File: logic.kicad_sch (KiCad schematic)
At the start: 41 parts, among them J4 Conn_01x04, J5 Conn_01x04, J6 Conn_01x04_Pin, J7 TC2030, SW1 SW_Push, SW2 SW_Push, U6 SN65HVD230, U7 HT753-1, U8 STM32F103C8Tx, Y1 8M

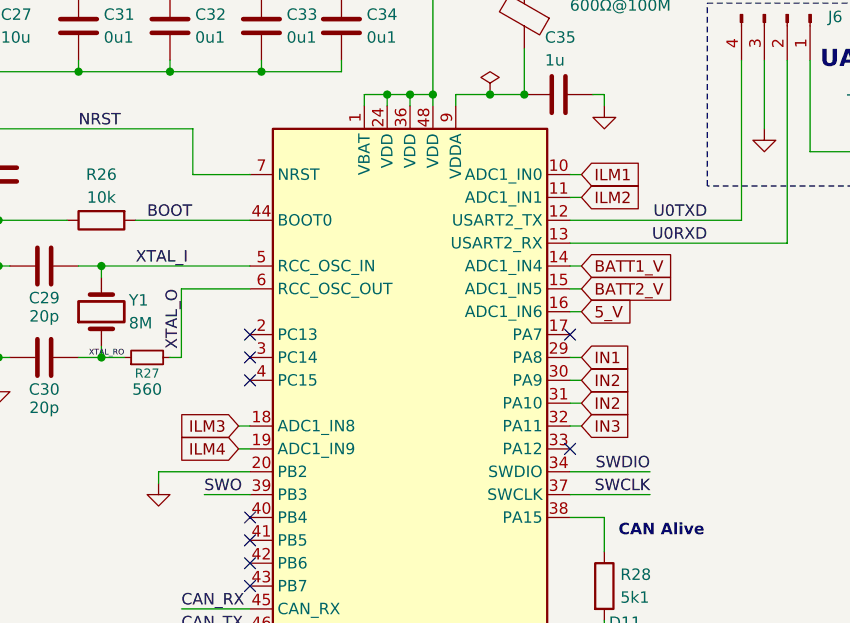
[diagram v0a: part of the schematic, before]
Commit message: pcb: add v and i routing
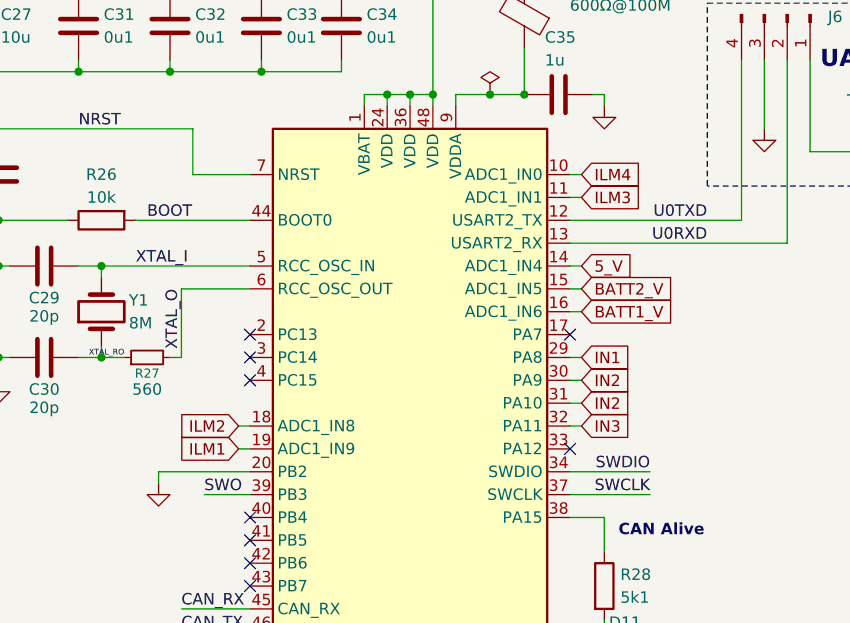
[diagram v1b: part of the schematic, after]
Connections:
- net 5_V: now also U8.14 (PA4); no longer U8.16 (PA6)
- net BATT1_V: now also U8.16 (PA6); no longer U8.14 (PA4)
- net ILM1: now also U8.19 (PB1); no longer U8.10 (PA0)
- net ILM2: now also U8.18 (PB0); no longer U8.11 (PA1)
- net ILM3: now also U8.11 (PA1); no longer U8.18 (PB0)
- net ILM4: now also U8.10 (PA0); no longer U8.19 (PB1)
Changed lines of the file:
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@@
+		)
+	)
+	(global_label "BATT1_V"
+		(shape input)
+		(at 161.29 77.47 0)
+		(fields_autoplaced yes)
+		(effects
+			(font
+				(size 1.27 1.27)
+			)
+			(justify left)
+		)
+		(property "Intersheetrefs" "${INTERSHEET_REFS}"
+			(at 171.8347 77.47 0)
+			(hide yes)
+			(show_name no)
+			(do_not_autoplace no)
+			(effects
+				(font
+					(size 1.27 1.27)
+				)
+				(justify left)
+			)
+		)
+	)
+	(global_label "ILM3"
+		(shape input)
+		(at 161.29 64.77 0)
+		(fields_autoplaced yes)
+		(effects
+			(font
+				(size 1.27 1.27)
+			)
+			(justify left)
+		)
+		(property "Intersheetrefs" "${INTERSHEET_REFS}"
+			(at 168.569 64.77 0)
+			(hide yes)
+			(show_name no)
+			(do_not_autoplace no)
+			(effects
+				(font
+					(size 1.27 1.27)
+				)
+				(justify left)
+			)
+		)
+	)
+	(global_label "ILM4"
+		(shape input)
+		(at 161.29 62.23 0)
+		(fields_autoplaced yes)
+		(effects
+			(font
+				(size 1.27 1.27)
+			)
+			(justify left)
+		)
+		(property "Intersheetrefs" "${INTERSHEET_REFS}"
+			(at 168.569 62.23 0)
+			(hide yes)
+			(show_name no)
+			(do_not_autoplace no)
+			(effects
+				(font
+					(size 1.27 1.27)
+				)
+				(justify left)
+			)
+		)
+	)
+	(global_label "ILM2"
+		(shape input)
+		(at 123.19 90.17 180)
+		(fields_autoplaced yes)
+		(effects
+			(font
+				(size 1.27 1.27)
+			)
+			(justify right)
+		)
+		(property "Intersheetrefs" "${INTERSHEET_REFS}"
+			(at 115.911 90.17 0)
+			(hide yes)
+			(show_name no)
+			(do_not_autoplace no)
+			(effects
+				(font
+					(size 1.27 1.27)
+				)
+				(justify right)
+			)
 		)
 	)
@@
 		)
 	)
-	(global_label "ILM2"
-		(shape input)
-		(at 161.29 64.77 0)
-		(fields_autoplaced yes)
-		(effects
-			(font
-				(size 1.27 1.27)
-			)
-			(justify left)
-		)
-		(property "Intersheetrefs" "${INTERSHEET_REFS}"
-			(at 168.569 64.77 0)
-			(hide yes)
-			(show_name no)
-			(do_not_autoplace no)
-			(effects
-				(font
-					(size 1.27 1.27)
-				)
-				(justify left)
-			)
-		)
-	)
-	(global_label "BATT1_V"
+	(global_label "5_V"
 		(shape input)
 		(at 161.29 72.39 0)
@@
 		)
 		(property "Intersheetrefs" "${INTERSHEET_REFS}"
-			(at 171.8347 72.39 0)
+			(at 167.5409 72.39 0)
+			(hide yes)
+			(show_name no)
+			(do_not_autoplace no)
+			(effects
+				(font
+					(size 1.27 1.27)
+				)
+				(justify left)
+			)
+		)
+	)
+	(global_label "IN1"
+		(shape input)
+		(at 161.29 82.55 0)
+		(fields_autoplaced yes)
+		(effects
+			(font
+				(size 1.27 1.27)
+			)
+			(justify left)
+		)
+		(property "Intersheetrefs" "${INTERSHEET_REFS}"
+			(at 167.42 82.55 0)
+			(hide yes)
+			(show_name no)
+			(do_not_autoplace no)
+			(effects
+				(font
+					(size 1.27 1.27)
+				)
+				(justify left)
+			)
+		)
+	)
+	(global_label "IN2"
+		(shape input)
+		(at 161.29 85.09 0)
+		(fields_autoplaced yes)
+		(effects
+			(font
+				(size 1.27 1.27)
+			)
+			(justify left)
+		)
+		(property "Intersheetrefs" "${INTERSHEET_REFS}"
+			(at 167.42 85.09 0)
 			(hide yes)
 			(show_name no)
@@
 	(global_label "ILM1"
 		(shape input)
-		(at 161.29 62.23 0)
-		(fields_autoplaced yes)
-		(effects
-			(font
-				(size 1.27 1.27)
-			)
-			(justify left)
-		)
-		(property "Intersheetrefs" "${INTERSHEET_REFS}"
-			(at 168.569 62.23 0)
-			(hide yes)
-			(show_name no)
-			(do_not_autoplace no)
-			(effects
-				(font
-					(size 1.27 1.27)
-				)
-				(justify left)
-			)
-		)
-	)
-	(global_label "IN1"
-		(shape input)
-		(at 161.29 82.55 0)
-		(fields_autoplaced yes)
-		(effects
-			(font
-				(size 1.27 1.27)
-			)
-			(justify left)
-		)
-		(property "Intersheetrefs" "${INTERSHEET_REFS}"
-			(at 167.42 82.55 0)
-			(hide yes)
-			(show_name no)
-			(do_not_autoplace no)
-			(effects
-				(font
-					(size 1.27 1.27)
-				)
-				(justify left)
-			)
-		)
-	)
-	(global_label "ILM4"
-		(shape input)
 		(at 123.19 92.71 180)
 		(fields_autoplaced yes)
@@
 			)
 		)
-	)
-	(global_label "IN2"
-		(shape input)
-		(at 161.29 85.09 0)
-		(fields_autoplaced yes)
-		(effects
-			(font
-				(size 1.27 1.27)
-			)
-			(justify left)
-		)
-		(property "Intersheetrefs" "${INTERSHEET_REFS}"
-			(at 167.42 85.09 0)
-			(hide yes)
-			(show_name no)
-			(do_not_autoplace no)
-			(effects
-				(font
-					(size 1.27 1.27)
-				)
-				(justify left)
-			)
-		)
-	)
-	(global_label "ILM3"
-		(shape input)
-		(at 123.19 90.17 180)
-		(fields_autoplaced yes)
-		(effects
-			(font
-				(size 1.27 1.27)
-			)
-			(justify right)
-		)
-		(property "Intersheetrefs" "${INTERSHEET_REFS}"
-			(at 115.911 90.17 0)
-			(hide yes)
-			(show_name no)
-			(do_not_autoplace no)
-			(effects
-				(font
-					(size 1.27 1.27)
-				)
-				(justify right)
-			)
-		)
-	)
-	(global_label "5_V"
-		(shape input)
-		(at 161.29 77.47 0)
-		(fields_autoplaced yes)
-		(effects
-			(font
-				(size 1.27 1.27)
-			)
-			(justify left)
-		)
-		(property "Intersheetrefs" "${INTERSHEET_REFS}"
-			(at 167.5409 77.47 0)
-			(hide yes)
-			(show_name no)
-			(do_not_autoplace no)
-			(effects
-				(font
-					(size 1.27 1.27)
-				)
-				(justify left)
-			)
-		)
